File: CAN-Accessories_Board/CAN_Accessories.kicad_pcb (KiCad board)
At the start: 2 copper layers, 83.8 x 63.5 mm, 47 parts, among them J1 39301040, J2 39301040, J3 39301040, J4 39301040, J5 39301040, J6 39301040, J7 39301060, J8 39301060, Q1 Q_NMOS_SGD, Q2 Q_NMOS_SGD, Q3 Q_NMOS_SGD, Q4 Q_NMOS_SGD, Q5 Q_NMOS_SGD, Q6 Q_NMOS_SGD, U1 NUCLEO_L432KC, U2 MCP2562FD-E_SN

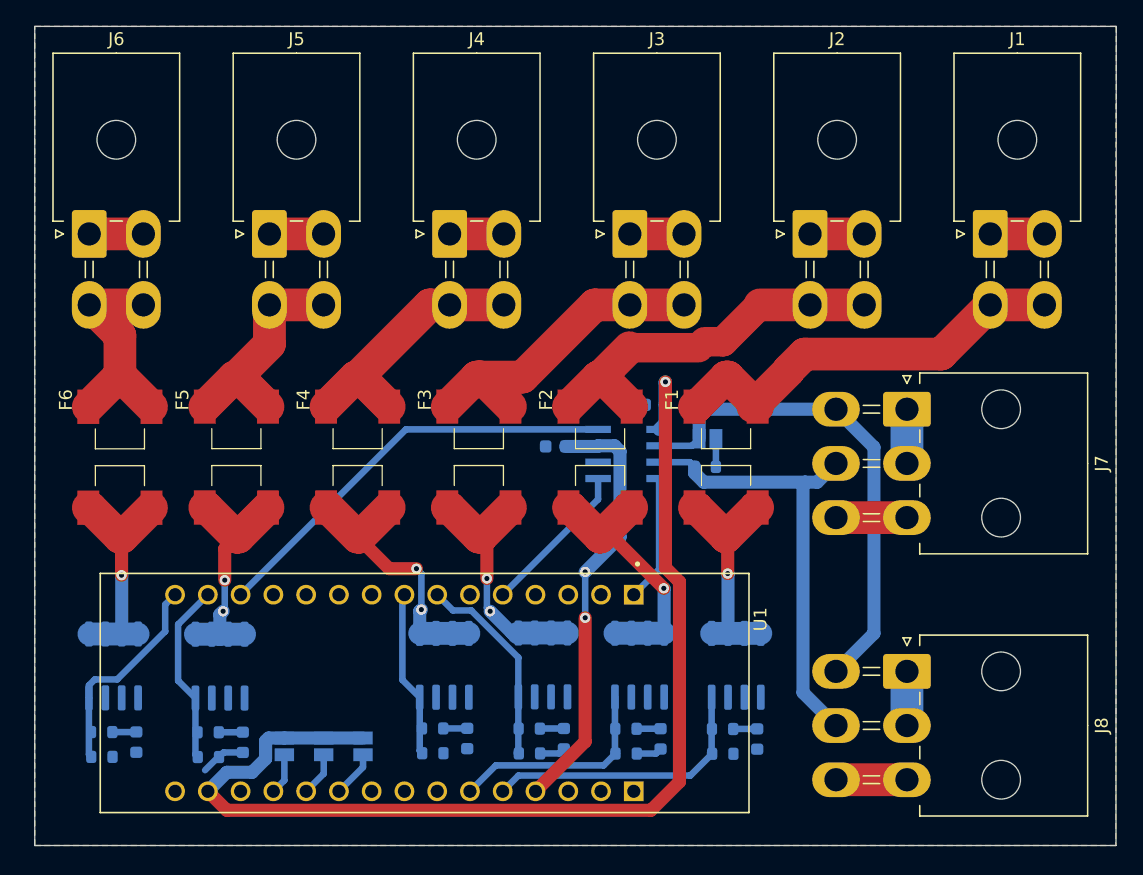
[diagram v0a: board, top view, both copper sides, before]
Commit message: Changed layout
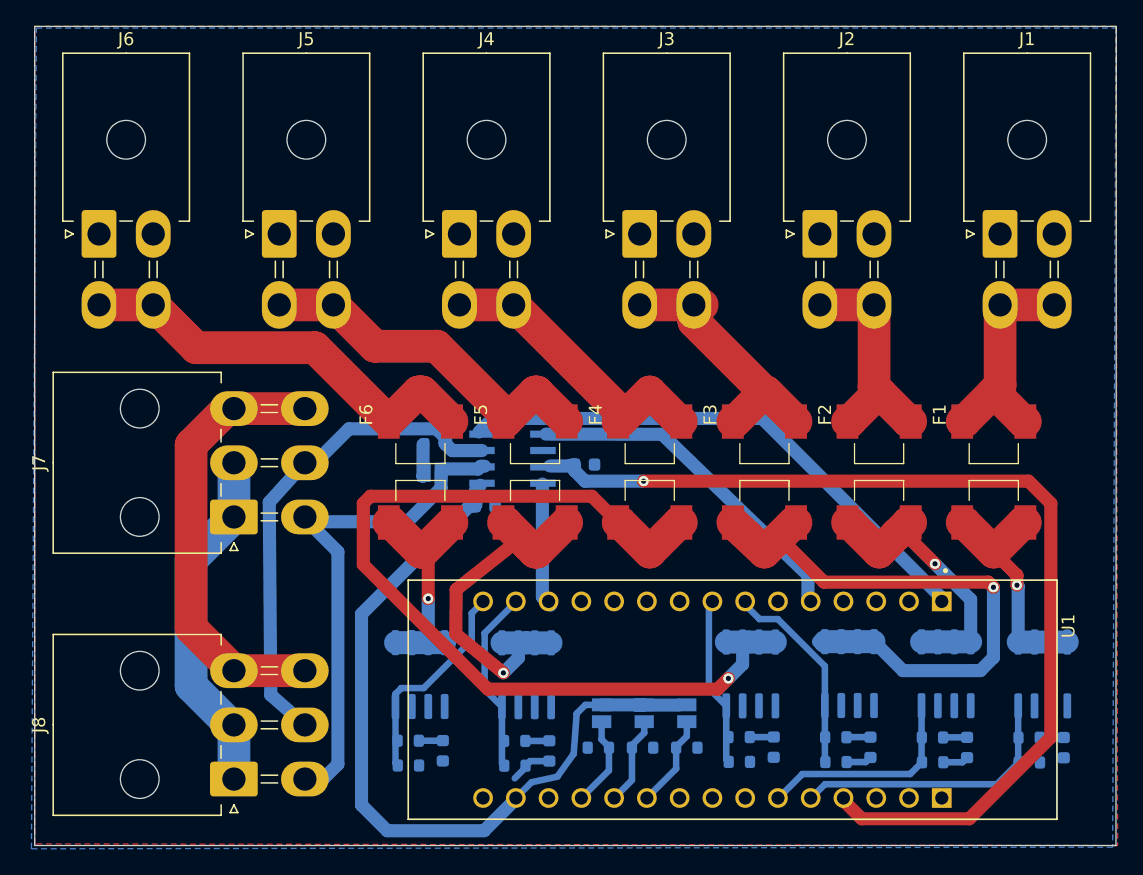
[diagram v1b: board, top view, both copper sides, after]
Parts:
- added R14: 10K, Resistor_SMD:R_0603_1608Metric, B.Cu at (88.7, 122.0)
- added R15: 10K, Resistor_SMD:R_0603_1608Metric, B.Cu at (85.2, 122.0)
- added R16: 10K, Resistor_SMD:R_0603_1608Metric, B.Cu at (81.8, 122.0)
- moved J7 52.8 mm to (53.5, 104.1), turned to 90 degrees
- moved J8 52.8 mm to (53.5, 124.4), turned to 90 degrees
- moved JP1 25.2 mm to (88.7, 119.3)
- moved JP2 25.0 mm to (85.3, 119.3)
- moved JP3 24.7 mm to (82.0, 119.3)
- moved U1 23.9 mm to (92.2, 118.2)
- moved D6 23.8 mm to (69.7, 122.2)
- moved R9 23.8 mm to (75.3, 121.4)
- moved D1 23.8 mm to (117.9, 122.0)
- moved D2 23.8 mm to (110.4, 121.9)
- moved D3 23.8 mm to (102.9, 121.9)
- moved D4 23.8 mm to (95.4, 121.9)
- moved D5 23.8 mm to (78.0, 122.2)
- moved Q1 23.8 mm to (116.2, 116.2)
- moved Q2 23.8 mm to (108.8, 116.2)
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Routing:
- net Net-(F4-Pad2): track 21.4 -> 72.1 mm, vias 2 -> 1
- net /5V: track 33.5 -> 77.6 mm, vias 2 -> 1
- net /STBY: track 9.82 -> 42.5 mm
- net /3V3: track 88.0 -> 60.3 mm, vias 1 -> 0
- net Net-(F3-Pad2): track 19.6 -> 46.6 mm, vias 2 -> 1
- net /CANRX: track 33.0 -> 9.65 mm
- net GND: track 18.5 -> 41.7 mm
- net Net-(F6-Pad1): track 17.6 -> 33.0 mm
- net /CANTX: track 12.1 -> 27.0 mm
- net Net-(F1-Pad1): track 32.7 -> 18.0 mm
- net Net-(F2-Pad1): track 28.9 -> 17.9 mm
- net Net-(F5-Pad1): track 17.7 -> 28.3 mm
- net Net-(F5-Pad2): track 18.7 -> 28.4 mm, vias 2 -> 1
- net +12V: track 33.6 -> 27.4 mm
- net Net-(F3-Pad1): track 25.0 -> 20.7 mm
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
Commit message: Changed PCB Layout
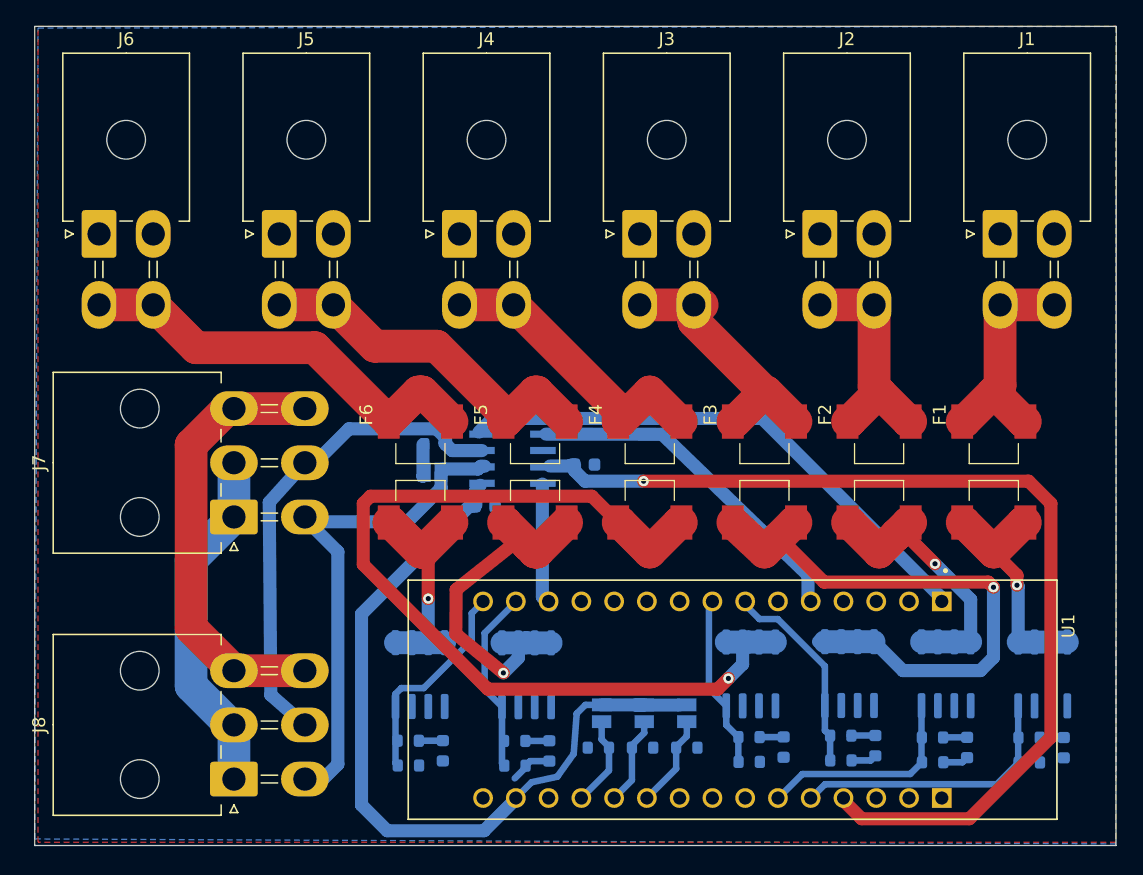
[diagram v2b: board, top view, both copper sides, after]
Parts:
- moved D4 0.76 mm to (96.2, 121.9)
- moved R7 0.76 mm to (93.5, 121.1)
- moved R8 0.76 mm to (93.5, 123.1)
- moved D3 0.40 mm to (103.3, 121.8)
- moved R5 0.40 mm to (100.6, 121.0)
- moved R6 0.40 mm to (100.6, 122.9)
